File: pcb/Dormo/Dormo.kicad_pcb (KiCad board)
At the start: 4 copper layers, 229 x 39 mm, 120 parts, among them J2 USB_C_Receptacle_USB2.0_16P, J3 FPC, 6P, P=0.5mm, J4 Conn_01x02, Q1 AO3401A, U1 ESP32-C3, U2 MIC5504-3.3YM5, U3 BRCL4054BME, Y1 40MHz

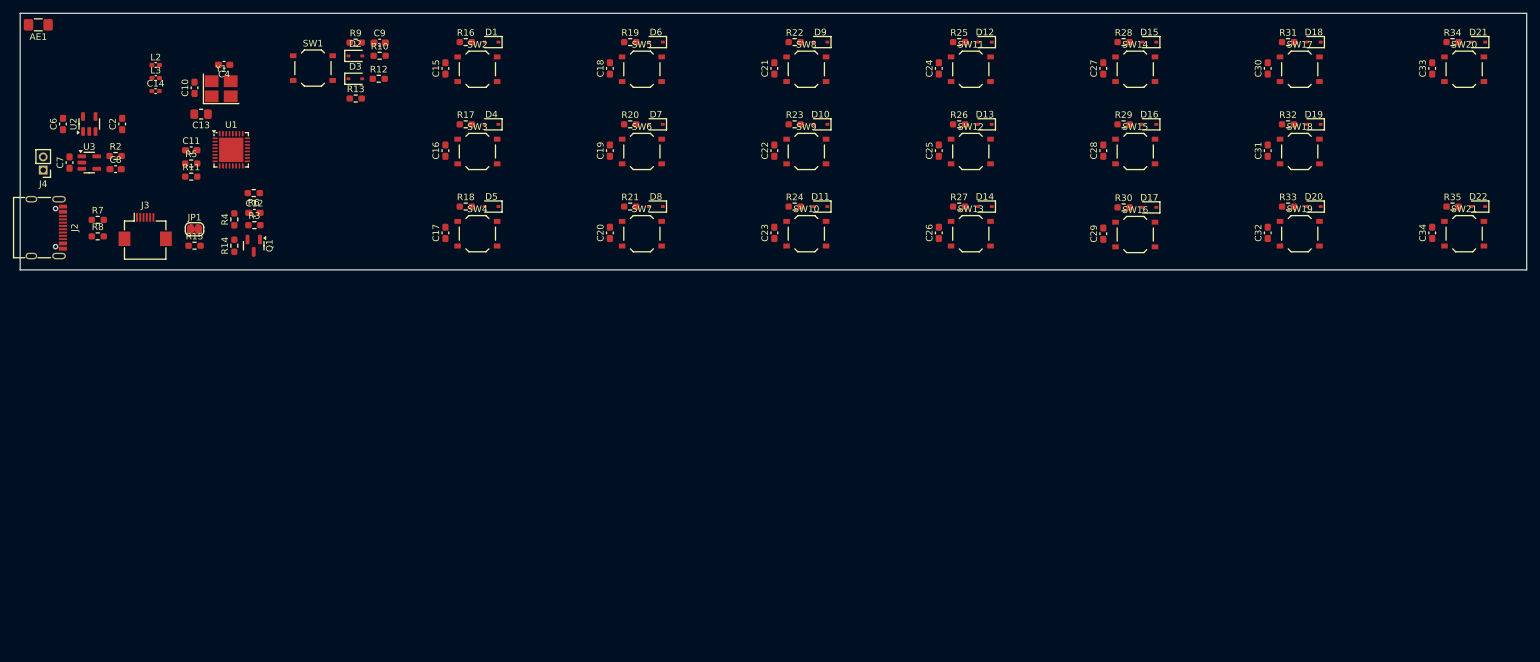
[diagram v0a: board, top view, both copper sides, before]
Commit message: minor layout tweaks
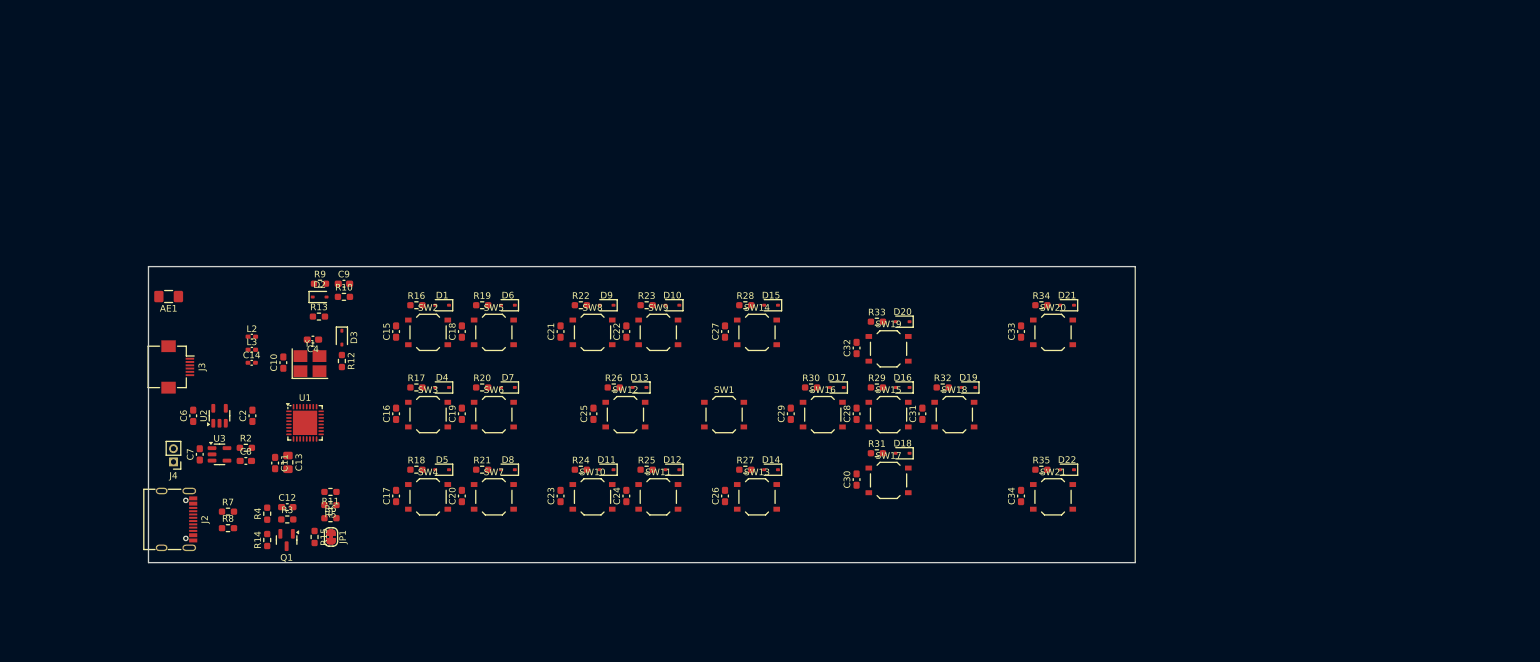
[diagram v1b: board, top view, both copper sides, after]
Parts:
- moved C30 88.4 mm to (157.6, 137.4)
- moved D18 88.4 mm to (164.6, 133.4)
- moved R31 88.4 mm to (160.7, 133.4)
- moved SW17 88.4 mm to (162.5, 137.5)
- moved SW1 81.7 mm to (137.5, 127.5)
- moved C24 80.5 mm to (122.6, 139.9)
- moved D12 80.5 mm to (129.6, 135.9)
- moved R25 80.5 mm to (125.7, 135.9)
- moved SW11 80.5 mm to (127.5, 140.0)
- moved C33 74.2 mm to (182.6, 114.9)
- moved C34 74.2 mm to (182.6, 139.9)
- moved D21 74.2 mm to (189.6, 110.9)
- moved D22 74.2 mm to (189.6, 135.9)
- moved R34 74.2 mm to (185.7, 110.9)
- moved R35 74.2 mm to (185.7, 135.9)
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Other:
- board size 229 x 39 mm -> 150 x 45 mm
- board text added: "Centerline"
- board text added: "Target size: approx 150mm x 45mm"
- board text removed: "Target size: approx 45mm x 150 mm"

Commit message: first pass of PCB routing
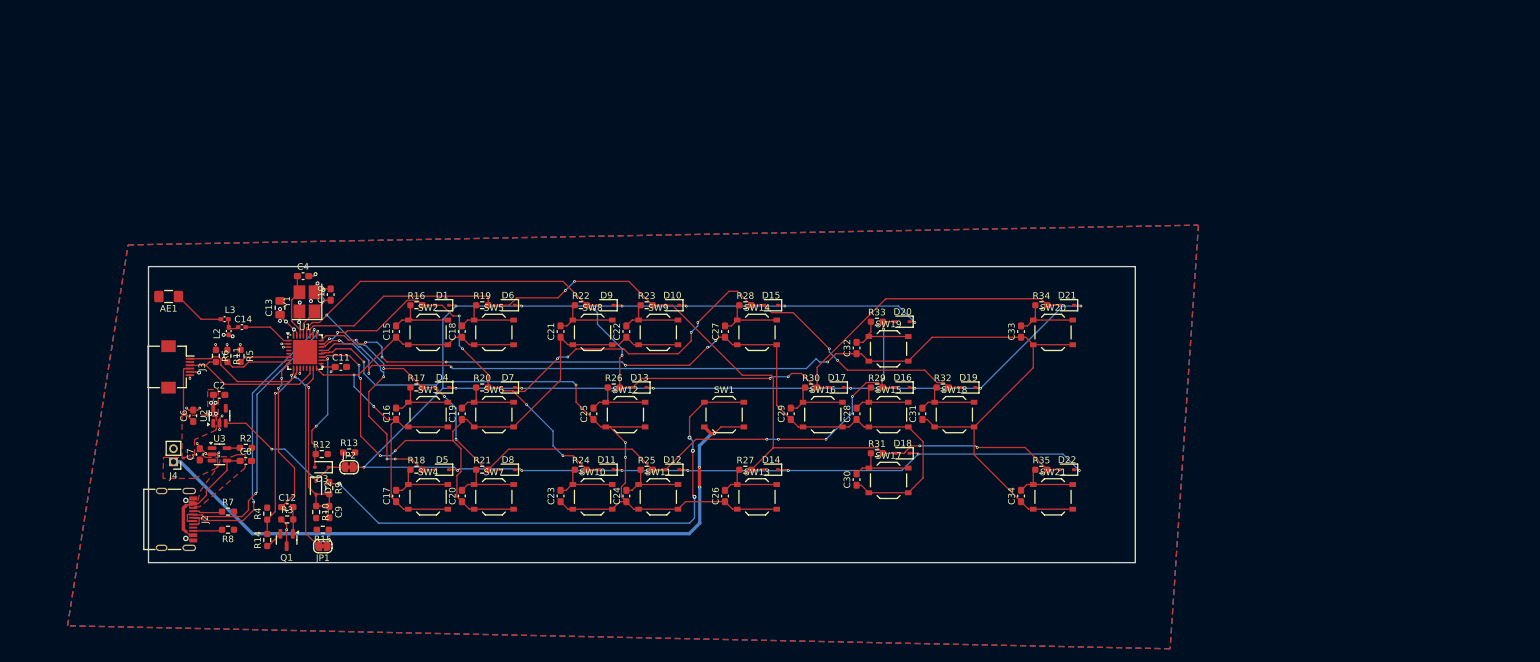
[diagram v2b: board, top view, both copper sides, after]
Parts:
- added JP2: Bridged, Jumper:SolderJumper-2_P1.3mm_Bridged_RoundedPad1.0x1.5mm, F.Cu at (80.5, 135.5)
- moved C9 34.8 mm to (77.5, 142.3), turned to -90 degrees
- moved R10 33.0 mm to (75.5, 142.3), turned to -90 degrees
- moved R9 31.1 mm to (77.5, 138.7), turned to -90 degrees
- moved R6 30.2 mm to (60.2, 118.6), turned to -90 degrees
- moved D2 29.0 mm to (75.5, 138.6), turned to -90 degrees
- moved R5 26.5 mm to (64.0, 118.6), turned to -90 degrees
- moved R11 25.9 mm to (62.0, 118.6), turned to -90 degrees
- moved C13 23.5 mm to (70.0, 111.2), turned to 90 degrees
- moved R13 21.2 mm to (80.5, 133.2)
- moved D3 19.9 mm to (76.3, 135.5), turned to 180 degrees
- moved C11 17.7 mm to (79.2, 120.2), turned to 0 degrees
- moved R12 14.5 mm to (76.3, 133.5), turned to 0 degrees
- moved C10 12.6 mm to (77.7, 109.2)
- moved U1 10.8 mm to (73.8, 118.0)
- moved C4 9.77 mm to (73.5, 106.5), turned to 0 degrees
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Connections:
- D1 pad 1: /LATCH -> /LATCH_MX
- D10 pad 1: /LATCH -> /LATCH_MX
- D11 pad 1: /LATCH -> /LATCH_MX
- D12 pad 1: /LATCH -> /LATCH_MX
- D13 pad 1: /LATCH -> /LATCH_MX
- D14 pad 1: /LATCH -> /LATCH_MX
- D15 pad 1: /LATCH -> /LATCH_MX
- D16 pad 1: /LATCH -> /LATCH_MX
- D17 pad 1: /LATCH -> /LATCH_MX
- D18 pad 1: /LATCH -> /LATCH_MX
- D19 pad 1: /LATCH -> /LATCH_MX
- D20 pad 1: /LATCH -> /LATCH_MX
- D21 pad 1: /LATCH -> /LATCH_MX
- D22 pad 1: /LATCH -> /LATCH_MX
- D4 pad 1: /LATCH -> /LATCH_MX
- D5 pad 1: /LATCH -> /LATCH_MX
- D6 pad 1: /LATCH -> /LATCH_MX
- D7 pad 1: /LATCH -> /LATCH_MX
- D8 pad 1: /LATCH -> /LATCH_MX
- D9 pad 1: /LATCH -> /LATCH_MX
- R9 pad 1: /LATCH -> Net-(R9-Pad1)
- SW1 pad 1: /LATCH -> Net-(R9-Pad1)
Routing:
- net /LATCH_MX: track 0.00 -> 339.1 mm, vias 0 -> 21
- net /COL_3: track 0.00 -> 179.6 mm, vias 0 -> 8
- net /GPIO15: track 0.00 -> 170.0 mm, vias 0 -> 4
- net /COL_4: track 0.00 -> 145.7 mm, vias 0 -> 4
- net /COL_1: track 0.00 -> 143.6 mm, vias 0 -> 12
- net /GPIO14: track 0.00 -> 126.1 mm, vias 0 -> 6
- net /COL_2: track 0.00 -> 123.4 mm, vias 0 -> 10
- net /+VBAT: track 0.00 -> 121.5 mm, vias 0 -> 4
- net /GPIO13: track 0.00 -> 106.5 mm, vias 0 -> 6
- net /GPIO12: track 0.00 -> 100.2 mm, vias 0 -> 4
- net Net-(R9-Pad1): track 0.00 -> 83.3 mm, vias 0 -> 4
- net /GPIO10: track 0.00 -> 74.3 mm, vias 0 -> 2
- net /BTN: track 0.00 -> 47.4 mm, vias 0 -> 2
- net /GPIO19: track 0.00 -> 45.2 mm, vias 0 -> 2
- net /GPIO18: track 0.00 -> 44.0 mm, vias 0 -> 2
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- added copper zone on F.Cu, net /+3V3
- added copper zone on In1.Cu, net /+3V3
- added copper zone on F.Cu, net /+VBAT
- added copper zone on F.Cu, net /+VUSB
- added copper zone on B.Cu, net GND
- added copper zone on F.Cu, net GND
- added copper zone on In2.Cu, net GND
